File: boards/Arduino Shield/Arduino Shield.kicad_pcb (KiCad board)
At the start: 2 copper layers, 115 x 75 mm, 22 parts, among them J1 Screw_Terminal_01x07, J11 Screw_Terminal_01x08, J2 Screw_Terminal_01x08, J3 Screw_Terminal_01x08, J4 Screw_Terminal_01x08, J5 Screw_Terminal_01x08, J6 Screw_Terminal_01x08, J7 Screw_Terminal_01x08, J8 Screw_Terminal_01x07, J9 Screw_Terminal_01x10, U1 A000062

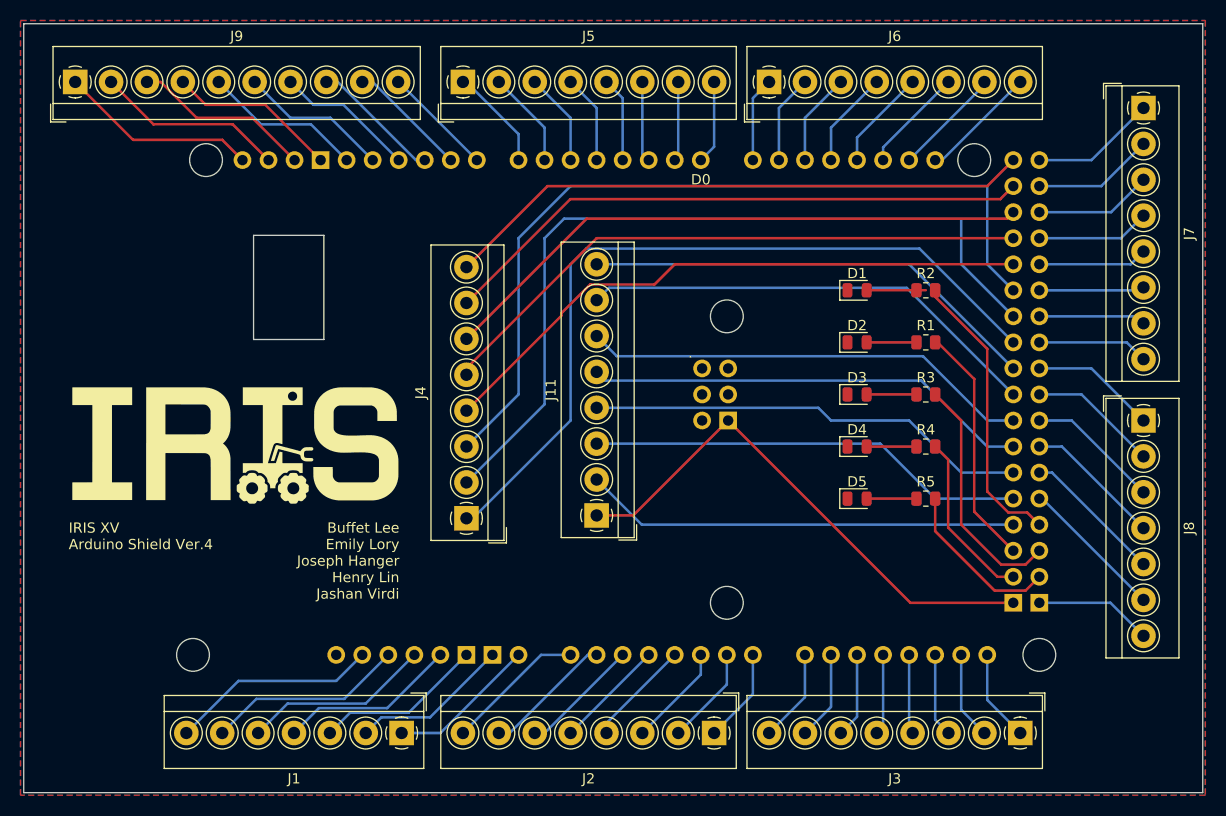
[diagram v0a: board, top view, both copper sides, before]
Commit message: Add labeling
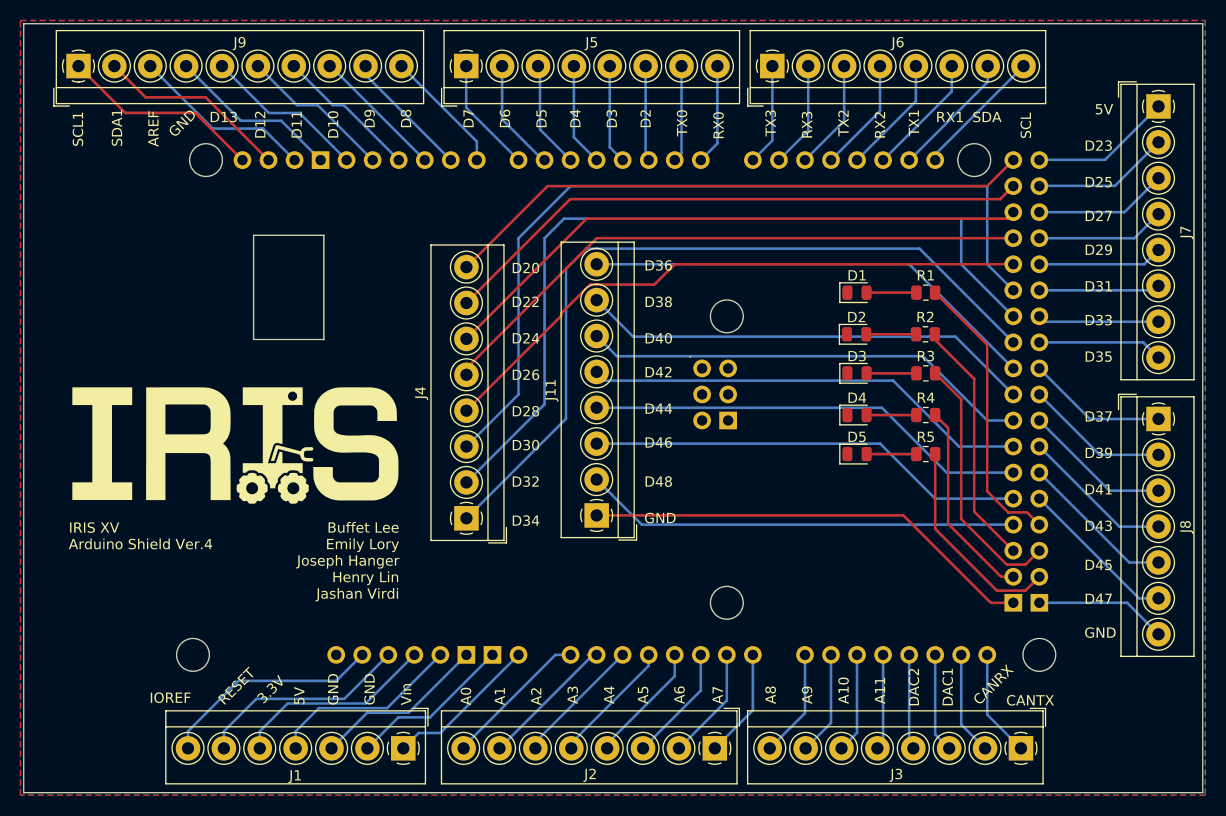
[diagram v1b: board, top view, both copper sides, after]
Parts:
- moved D5 4.34 mm to (101.3, 62.0)
- moved R5 4.34 mm to (108.0, 62.0)
- moved D4 3.07 mm to (101.3, 58.2)
- moved R4 3.07 mm to (108.0, 58.2)
- moved D3 2.06 mm to (101.3, 54.1)
- moved R3 2.06 mm to (108.0, 54.1)
- moved J9 1.58 mm to (25.3, 24.1)
- moved J5 1.58 mm to (63.2, 24.1)
- moved J6 1.58 mm to (93.0, 24.1)
- moved J1 1.51 mm to (57.0, 90.7)
- moved J2 1.50 mm to (87.4, 90.7)
- moved J3 1.50 mm to (117.3, 90.7)
- moved J8 1.47 mm to (130.7, 58.5)
- moved J7 1.47 mm to (130.7, 28.1)
- moved D2 0.79 mm to (101.2, 50.3)
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- renumbered R2 to R1, R1 to R2
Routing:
- net GND: track 111.9 -> 106.9 mm
- net Net-(U1-D53): track 16.3 -> 20.5 mm
- net Net-(U1-D52): track 16.8 -> 19.6 mm
- net Net-(J6-Pin_8): track 11.5 -> 13.4 mm
- net Net-(U1-D51): track 23.5 -> 25.3 mm
- net Net-(J6-Pin_7): track 10.7 -> 12.4 mm
- net Net-(J6-Pin_6): track 10.3 -> 11.9 mm
- net Net-(J6-Pin_5): track 9.87 -> 11.5 mm
- net Net-(J6-Pin_2): track 8.67 -> 10.4 mm
- net Net-(J6-Pin_1): track 8.27 -> 9.96 mm
- net Net-(J5-Pin_7): track 7.76 -> 9.44 mm
- net Net-(J6-Pin_4): track 9.47 -> 11.1 mm
- net Net-(J6-Pin_3): track 9.07 -> 10.8 mm
- net Net-(J5-Pin_8): track 8.16 -> 9.84 mm
- net Net-(J8-Pin_6): track 14.3 -> 15.9 mm
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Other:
- board text added: "3.3V"
- board text added: "5V"
- board text added: "A0"
- board text added: "A1"
- board text added: "A10"
- board text added: "A11"
- board text added: "A2"
- board text added: "A3"
- board text added: "A4"
- board text added: "A5"
- board text added: "A6"
- board text added: "A7"
- board text added: "A8"
- board text added: "A9"
- board text added: "AREF"
- board text added: "CANRX"
- board text added: "CANTX"
- board text added: "D10"
- board text added: "D11"
- board text added: "D12"
- board text added: "D13"
- board text added: "D2"
- board text added: "D20"
- board text added: "D22"
- board text added: "D23"
- board text added: "D24"
- board text added: "D25"
- board text added: "D26"
- board text added: "D27"
- board text added: "D28"
- board text added: "D29"
- board text added: "D3"
- board text added: "D30"
- board text added: "D31"
- board text added: "D32"
- board text added: "D33"
- board text added: "D34"
- board text added: "D35"
- board text added: "D36"
- board text added: "D37"
- board text added: "D38"
- board text added: "D39"
- board text added: "D4"
- board text added: "D40"
- board text added: "D41"
- board text added: "D42"
- board text added: "D43"
- board text added: "D44"
- board text added: "D45"
- board text added: "D46"
- board text added: "D47"
- board text added: "D48"
- board text added: "D5"
- board text added: "D6"
- board text added: "D7"
- board text added: "D8"
- board text added: "D9"
- board text added: "DAC1"
- board text added: "DAC2"
- board text added: "GND"
- board text added: "IOREF"
- board text added: "JLCJLCJLCJLC"
- board text added: "RESET"
- board text added: "RX0"
- board text added: "RX1"
- board text added: "RX2"
- board text added: "RX3"
- board text added: "SCL"
- board text added: "SCL1"
- board text added: "SDA"
- board text added: "SDA1"
- board text added: "TX0"
- board text added: "TX1"
- board text added: "TX2"
- board text added: "TX3"
- board text added: "Vin"
